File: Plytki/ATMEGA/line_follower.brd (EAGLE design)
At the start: 25.1 x 25.4 mm, 5 parts

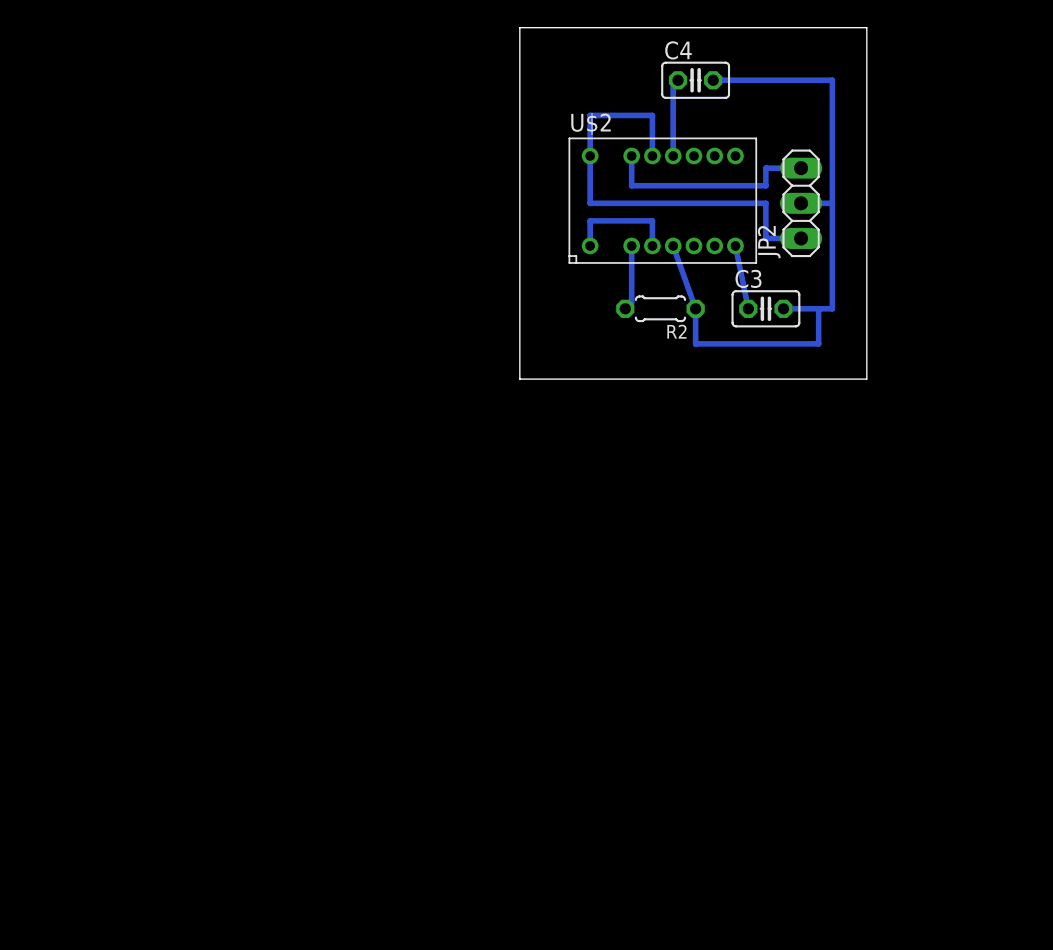
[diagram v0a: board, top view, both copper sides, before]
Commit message: Ostateczne projekty plytek
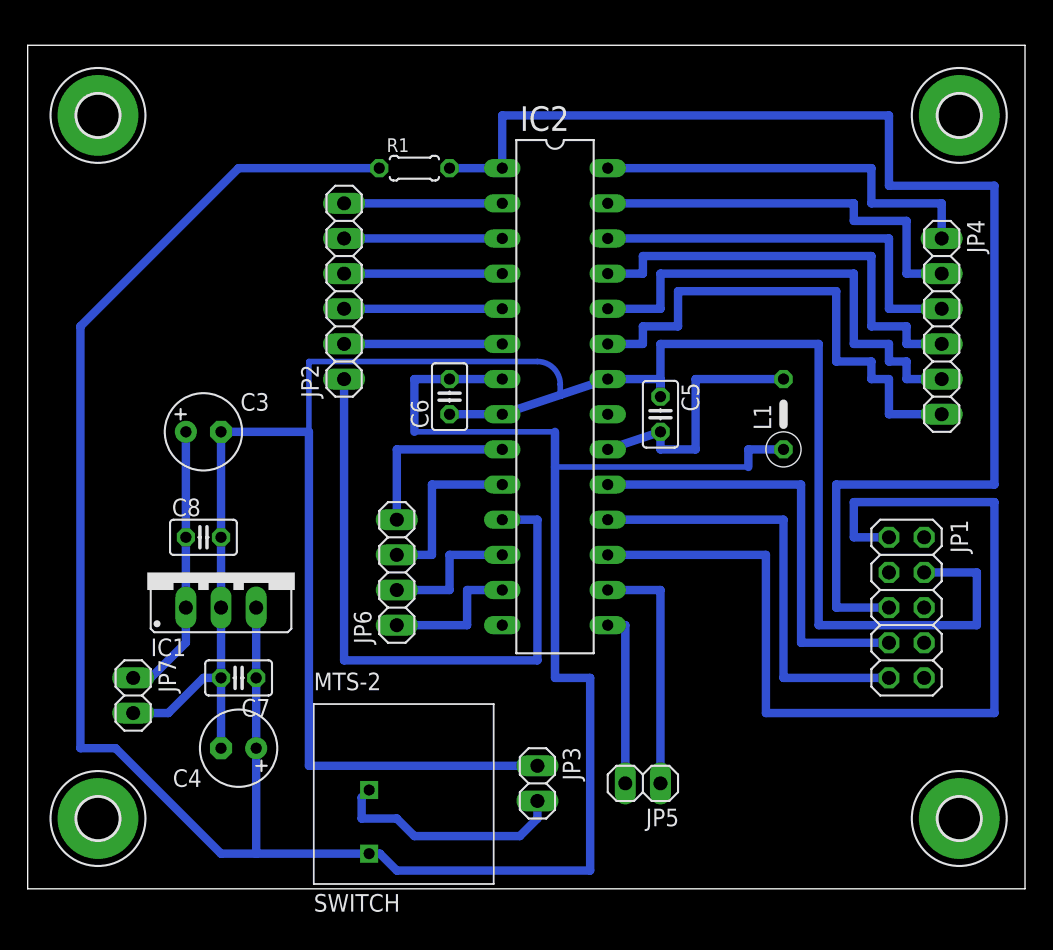
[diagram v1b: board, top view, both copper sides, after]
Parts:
- removed R2: (no value), rcl:0204/5
- removed U$2: (no value), SharpGP2Y0D810Z0F:LP16PIN
- added C5, C7, C8: 100nF, rcl:C025-025X050
- added C6: (no value), rcl:C025-025X050
- added H1, H2, H3, H4: MOUNT-PAD-ROUND3.0, holes:3,0-PAD
- added IC1: (no value), v-reg:78XXS
- added IC2: MEGA8-P, atmel:DIL28-3
- added JP1: (no value), pinhead:2X05
- added JP3, JP5, JP7: (no value), pinhead:1X02
- added JP4: (no value), pinhead:1X06
- added JP6: (no value), pinhead:1X04
- added L1: 10uH, rcl:0207/5V
- added MTS-2: SWITCH, MTS-2:MTS-2_SWITCH
- added R1: 1k, rcl:0204/5
- C3, C4: value 0.1 μF -> 470uF; device rcl:C025-025X050 -> rcl:E2,5-6
- JP2: device pinhead:1X03 -> pinhead:1X06
- moved C4 58.5 mm to (15.2, 10.2), turned to 180 degrees
- moved C3 41.6 mm to (12.7, 33.0)
- moved JP2 33.6 mm to (22.9, 43.2)
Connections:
- removed net VCC: C4.1, JP2.1, U$2.11, U$2.12, U$2.14
- new net +5V: C4.+, C6.2, C7.1, IC1.OUT, IC2.7, L1.1, MTS-2.PIN1, R1.1
- new net LP: IC2.9, JP6.4
- new net LT: IC2.10, JP6.3
- new net N$1: C5.2, IC2.20, L1.2
- new net N$10: IC2.5, JP2.3
- new net N$11: IC2.6, JP2.2
- new net N$12: IC2.11, JP2.1
- new net N$13: C3.+, C8.1, IC1.IN, JP7.1
- new net N$14: IC2.24, JP4.5
- new net N$15: IC2.25, JP4.4
- new net N$16: IC2.26, JP4.3
- new net N$17: IC2.27, JP4.2
- new net N$18: IC2.28, JP4.1
- new net N$19: IC2.15, JP5.2
- new net N$2: IC2.23, JP4.6
- new net N$20: IC2.16, JP5.1
- new net N$22: JP3.2, MTS-2.PIN2
- new net N$3: IC2.1, JP1.5, R1.2
- new net N$4: IC2.17, JP1.1
- new net N$9: IC2.4, JP2.4
- new net PP: IC2.12, JP6.2
- new net PT: IC2.13, JP6.1
- net GND: now also C3.-, C4.-, C5.1, C6.1, C7.2, C8.2, IC1.GND, IC2.22, IC2.8, JP1.4, JP3.1, JP7.2; no longer C3.2, C4.2, JP2.2, R2.1, U$2.4
- net N$5: now also IC2.18, JP1.9; no longer R2.2, U$2.2
- net N$6: now also IC2.2, JP2.6; no longer C3.1, U$2.7
- net N$7: now also IC2.19, JP1.7; no longer U$2.1, U$2.3
- net N$8: now also IC2.3, JP2.5; no longer JP2.3, U$2.13
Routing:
- net +5V: track 0.00 -> 187.4 mm
- net GND: track 49.7 -> 173.5 mm
- net N$3: track 0.00 -> 94.0 mm
- net N$4: track 0.00 -> 69.8 mm
- net N$12: track 0.00 -> 47.0 mm
- net VCC: track 37.4 -> 0.00 mm
- net N$2: track 0.00 -> 36.8 mm
- net N$14: track 0.00 -> 34.3 mm
- net N$15: track 0.00 -> 31.8 mm
- net N$16: track 0.00 -> 29.2 mm
- net N$18: track 0.00 -> 29.2 mm
- net N$17: track 0.00 -> 29.2 mm
- net N$5: track 4.73 -> 31.8 mm
- net N$7: track 8.12 -> 31.8 mm
- net N$13: track 0.00 -> 20.1 mm
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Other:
- board size 25.1 x 25.4 mm -> 72.1 x 61 mm
